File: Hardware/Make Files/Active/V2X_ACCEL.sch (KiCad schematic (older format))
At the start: 7 parts, among them P25 CONN_02X08, U19 ADXL345

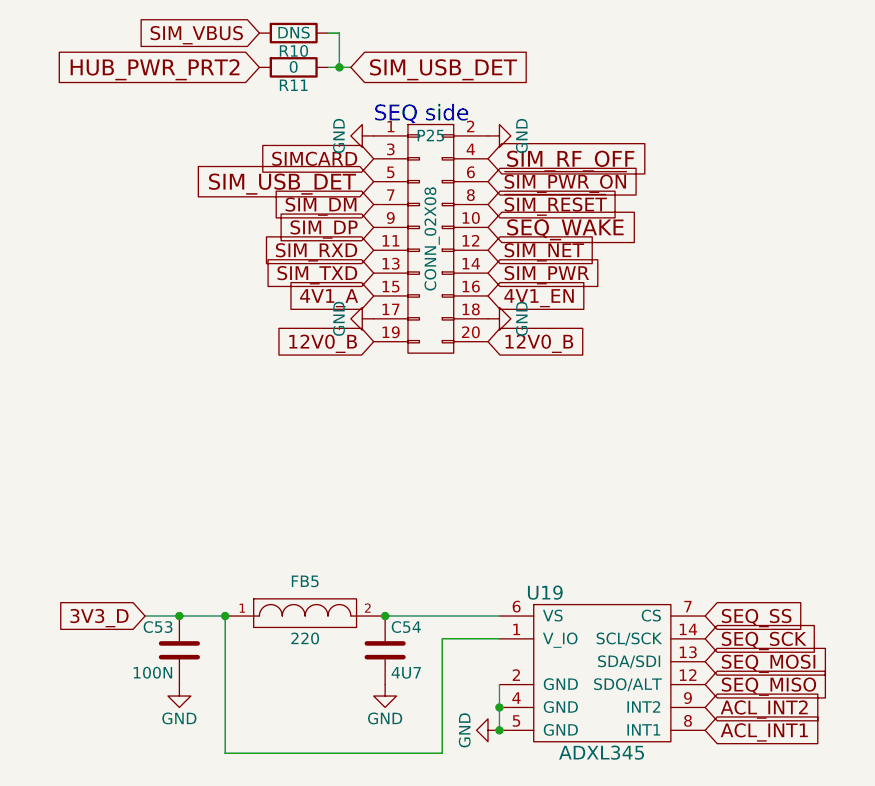
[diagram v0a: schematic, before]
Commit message: work from home day
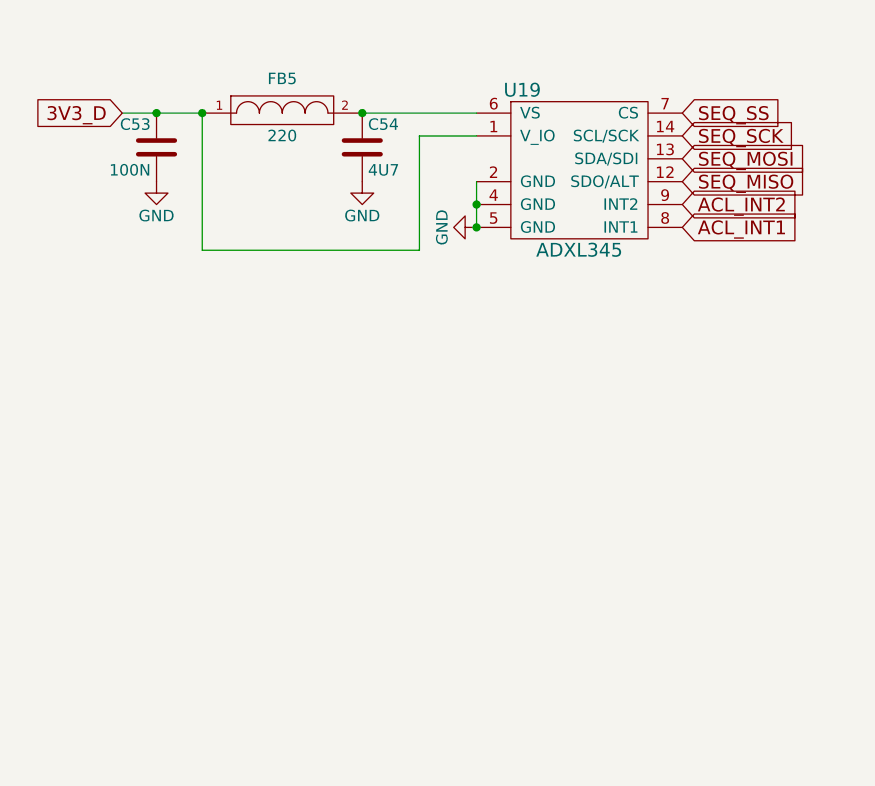
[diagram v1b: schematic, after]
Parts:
- removed P25: CONN_02X08, Pin_Headers:Pin_Header_Straight_2x10, symbol CONN_02X10
- removed R10: DNS, Custom Parts:R_0603_sm, symbol R
- removed R11: 0, Custom Parts:R_0603_sm, symbol R
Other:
- note removed: "SEQ side"
- moved on the sheet: C53, C54, FB5, U19

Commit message: BOM updates
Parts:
- C54: Mouse PN 963-LMK212B7475KG-T -> 581-12063C475KAT2A
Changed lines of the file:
@@
 F 2 "Custom Parts:C_0805_SM" H 2488 1300 30  0001 C CNN
 F 3 "http://www.yuden.co.jp/productdata/catalog/en/mlcc_all_e.pdf" H 2450 1450 60  0001 C CNN
-F 4 "963-LMK212B7475KG-T" H 2450 1450 60  0001 C CNN "Mouse PN"
+F 4 "581-12063C475KAT2A" H 2450 1450 60  0001 C CNN "Mouse PN"
 	1    2450 1450
 	1    0    0    -1
